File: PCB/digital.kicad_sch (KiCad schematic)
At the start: 34 parts, among them J13 JTAG, J14 FINAL_CARRERA_UP, J15 FINAL_CARRERA_DOWN, J3 ICSP, J4 CAN, J6 USART, J7 SPI, J8 RFID_COAX, U2 PIC32MK0256MCJ048-I/Y8X, U3 TCAN334D, Y1 ECS-3225SMV-080-GP-TR, Y2 ECS-3225SMV-080-GP-TR

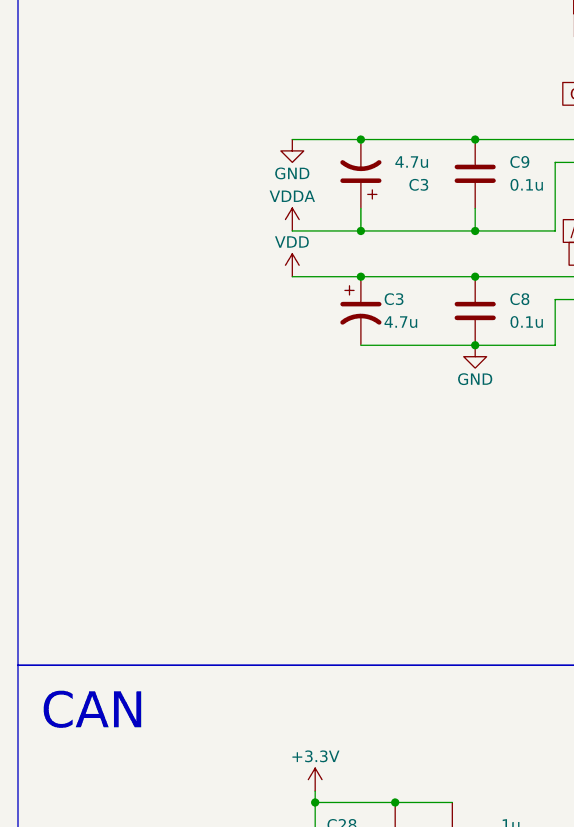
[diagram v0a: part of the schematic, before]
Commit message: start digital
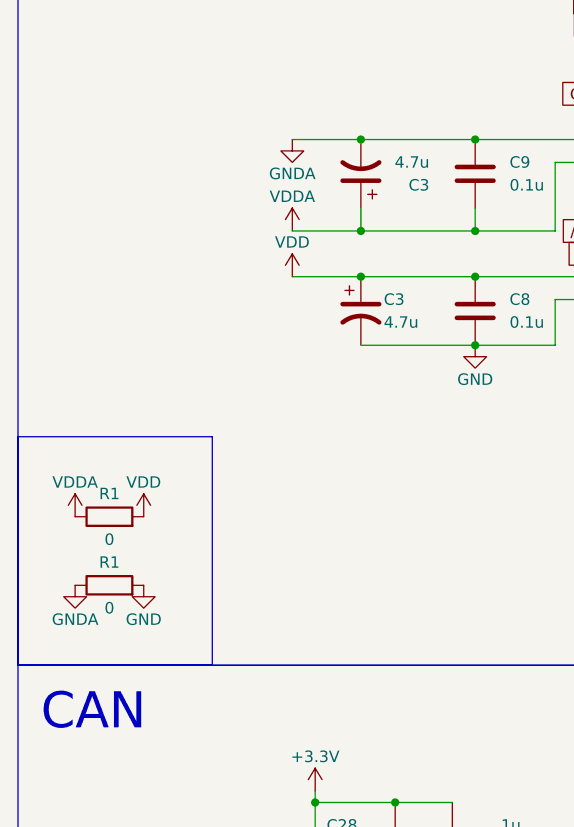
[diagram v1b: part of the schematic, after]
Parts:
- added R1 (x2): 0, symbol Device:R
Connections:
- net GND: now also R1.2; no longer C3.2, C9.1, U2.16 (AVSS)
- net VDD: now also R1.2
- net VDDA: now also R1.1
- new net GNDA: C3.2, C9.1, R1.1, U2.16 (AVSS)
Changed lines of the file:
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@@
+    (fill (type none))
+  )
+  (rectangle (start 12.7 104.14) (end 34.29 129.54)
+    (stroke (width 0) (type default))
     (fill (type none))
   )
@@
     )
   )
+  (symbol (lib_id "Device:R") (at 22.86 113.03 90) (unit 1)
+    (in_bom yes) (on_board yes) (dnp no)
+    (property "Reference" "R1" (at 22.86 110.49 90)
+      (effects (font (size 1.27 1.27)))
+    )
+    (property "Value" "0" (at 22.86 115.57 90)
+      (effects (font (size 1.27 1.27)))
+    )
+    (property "Footprint" "" (at 22.86 114.808 90)
+      (effects (font (size 1.27 1.27)) hide)
+    )
+    (property "Datasheet" "~" (at 22.86 113.03 0)
+      (effects (font (size 1.27 1.27)) hide)
+    )
+    (pin "1")
+    (pin "2")
+    (instances
+      (project "DIJOUS_4_PORTES"
+        (path "/69b34976-047e-478e-bd76-9b6ef0dba356/0e58b9bb-7a32-4563-ae50-f5e325ba8348"
+          (reference "R1") (unit 1)
+        )
+        (path "/69b34976-047e-478e-bd76-9b6ef0dba356/6b83d062-cc2b-4223-9dc9-bddc64623104"
+          (reference "R2") (unit 1)
+        )
+      )
+    )
+  )
+  (symbol (lib_id "power:VDDA") (at 19.05 113.03 0) (unit 1)
+    (in_bom yes) (on_board yes) (dnp no) (fields_autoplaced)
+    (property "Reference" "#PWR08" (at 19.05 116.84 0)
+      (effects (font (size 1.27 1.27)) hide)
+    )
+    (property "Value" "VDDA" (at 19.05 109.22 0)
+      (effects (font (size 1.27 1.27)))
+    )
+    (property "Footprint" "" (at 19.05 113.03 0)
+      (effects (font (size 1.27 1.27)) hide)
+    )
+    (property "Datasheet" "" (at 19.05 113.03 0)
+      (effects (font (size 1.27 1.27)) hide)
+    )
+    (pin "1")
+    (instances
+      (project "DIJOUS_4_PORTES"
+        (path "/69b34976-047e-478e-bd76-9b6ef0dba356/6b83d062-cc2b-4223-9dc9-bddc64623104"
+          (reference "#PWR08") (unit 1)
+        )
+      )
+    )
+  )
   (symbol (lib_id "Device:R") (at 39.37 31.75 270) (unit 1)
     (in_bom yes) (on_board yes) (dnp no)
@@
         (path "/69b34976-047e-478e-bd76-9b6ef0dba356/6b83d062-cc2b-4223-9dc9-bddc64623104"
           (reference "R4") (unit 1)
-        )
-      )
-    )
-  )
-  (symbol (lib_id "power:GND") (at 43.18 71.12 0) (unit 1)
-    (in_bom yes) (on_board yes) (dnp no)
-    (property "Reference" "#PWR015" (at 43.18 77.47 0)
-      (effects (font (size 1.27 1.27)) hide)
-    )
-    (property "Value" "GND" (at 43.18 74.93 0)
-      (effects (font (size 1.27 1.27)))
-    )
-    (property "Footprint" "" (at 43.18 71.12 0)
-      (effects (font (size 1.27 1.27)) hide)
-    )
-    (property "Datasheet" "" (at 43.18 71.12 0)
-      (effects (font (size 1.27 1.27)) hide)
-    )
-    (pin "1")
-    (instances
-      (project "DIJOUS_4_PORTES"
-        (path "/69b34976-047e-478e-bd76-9b6ef0dba356/6b83d062-cc2b-4223-9dc9-bddc64623104"
-          (reference "#PWR015") (unit 1)
         )
       )
@@
     )
   )
+  (symbol (lib_id "power:GNDA") (at 19.05 120.65 0) (unit 1)
+    (in_bom yes) (on_board yes) (dnp no)
+    (property "Reference" "#PWR07" (at 19.05 127 0)
+      (effects (font (size 1.27 1.27)) hide)
+    )
+    (property "Value" "GNDA" (at 19.05 124.46 0)
+      (effects (font (size 1.27 1.27)))
+    )
+    (property "Footprint" "" (at 19.05 120.65 0)
+      (effects (font (size 1.27 1.27)) hide)
+    )
+    (property "Datasheet" "" (at 19.05 120.65 0)
+      (effects (font (size 1.27 1.27)) hide)
+    )
+    (pin "1")
+    (instances
+      (project "DIJOUS_4_PORTES"
+        (path "/69b34976-047e-478e-bd76-9b6ef0dba356/6b83d062-cc2b-4223-9dc9-bddc64623104"
+          (reference "#PWR07") (unit 1)
+        )
+      )
+    )
+  )
   (symbol (lib_id "power:GND") (at 271.78 105.41 0) (unit 1)
     (in_bom yes) (on_board yes) (dnp no)
@@
         (path "/69b34976-047e-478e-bd76-9b6ef0dba356/6b83d062-cc2b-4223-9dc9-bddc64623104"
           (reference "C29") (unit 1)
+        )
+      )
+    )
+  )
+  (symbol (lib_id "power:GND") (at 26.67 120.65 0) (unit 1)
+    (in_bom yes) (on_board yes) (dnp no)
+    (property "Reference" "#PWR09" (at 26.67 127 0)
+      (effects (font (size 1.27 1.27)) hide)
+    )
+    (property "Value" "GND" (at 26.67 124.46 0)
+      (effects (font (size 1.27 1.27)))
+    )
+    (property "Footprint" "" (at 26.67 120.65 0)
+      (effects (font (size 1.27 1.27)) hide)
+    )
+    (property "Datasheet" "" (at 26.67 120.65 0)
+      (effects (font (size 1.27 1.27)) hide)
+    )
+    (pin "1")
+    (instances
+      (project "DIJOUS_4_PORTES"
+        (path "/69b34976-047e-478e-bd76-9b6ef0dba356/6b83d062-cc2b-4223-9dc9-bddc64623104"
+          (reference "#PWR09") (unit 1)
         )
       )
@@
         (path "/69b34976-047e-478e-bd76-9b6ef0dba356/6b83d062-cc2b-4223-9dc9-bddc64623104"
           (reference "J3") (unit 1)
+        )
+      )
+    )
+  )
+  (symbol (lib_id "power:VDD") (at 26.67 113.03 0) (unit 1)
+    (in_bom yes) (on_board yes) (dnp no)
+    (property "Reference" "#PWR015" (at 26.67 116.84 0)
+      (effects (font (size 1.27 1.27)) hide)
+    )
+    (property "Value" "VDD" (at 26.67 109.22 0)
+      (effects (font (size 1.27 1.27)))
+    )
+    (property "Footprint" "" (at 26.67 113.03 0)
+      (effects (font (size 1.27 1.27)) hide)
+    )
+    (property "Datasheet" "" (at 26.67 113.03 0)
+      (effects (font (size 1.27 1.27)) hide)
+    )
+    (pin "1")
+    (instances
+      (project "DIJOUS_4_PORTES"
+        (path "/69b34976-047e-478e-bd76-9b6ef0dba356/6b83d062-cc2b-4223-9dc9-bddc64623104"
+          (reference "#PWR015") (unit 1)
         )
       )
@@
         )
       )
+    )
+  )
+  (symbol (lib_id "power:GNDA") (at 43.18 71.12 0) (unit 1)
+    (in_bom yes) (on_board yes) (dnp no)
+    (property "Reference" "#PWR04" (at 43.18 77.47 0)
+      (effects (font (size 1.27 1.27)) hide)
+    )
+    (property "Value" "GNDA" (at 43.18 74.93 0)
+      (effects (font (size 1.27 1.27)))
+    )
+    (property "Footprint" "" (at 43.18 71.12 0)
+      (effects (font (size 1.27 1.27)) hide)
+    )
+    (property "Datasheet" "" (at 43.18 71.12 0)
+      (effects (font (size 1.27 1.27)) hide)
+    )
+    (pin "1")
+    (instances
+      (project "DIJOUS_4_PORTES"
+        (path "/69b34976-047e-478e-bd76-9b6ef0dba356/6b83d062-cc2b-4223-9dc9-bddc64623104"
+          (reference "#PWR04") (unit 1)
+        )
+      )
+    )
+  )
+  (symbol (lib_id "Device:R") (at 22.86 120.65 90) (unit 1)
+    (in_bom yes) (on_board yes) (dnp no)
+    (property "Reference" "R1" (at 22.86 118.11 90)
+      (effects (font (size 1.27 1.27)))
+    )
+    (property "Value" "0" (at 22.86 123.19 90)
+      (effects (font (size 1.27 1.27)))
+    )
+    (property "Footprint" "" (at 22.86 122.428 90)
+      (effects (font (size 1.27 1.27)) hide)
+    )
+    (property "Datasheet" "~" (at 22.86 120.65 0)
+      (effects (font (size 1.27 1.27)) hide)
+    )
+    (pin "1")
+    (pin "2")
+    (instances
+      (project "DIJOUS_4_PORTES"
+        (path "/69b34976-047e-478e-bd76-9b6ef0dba356/0e58b9bb-7a32-4563-ae50-f5e325ba8348"
+          (reference "R1") (unit 1)
+        )
+        (path "/69b34976-047e-478e-bd76-9b6ef0dba356/6b83d062-cc2b-4223-9dc9-bddc64623104"
+          (reference "R9") (unit 1)
+        )
+      )
